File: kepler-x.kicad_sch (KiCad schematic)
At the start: 60 parts, among them IC1 SLG46826G, J1 HDMI_C_1.3, J2 HDMI_A, J3 Jack_3.5mm_3pin, J4 RasPI_IO_Header_B+, SW1 SWITCH_INV, SW2 SWITCH_INV, U1 Bus-X68000-ext, U10 74AHC16374, U11 74LVTH162245, U12 TC7MPB9307F, U13 TC7MPB9307F, U14 P0082(DE0-NANO), U15 PLR135-T10, U16 PCM5102, U17 LT1117-3.3, U2 LT1117-3.3, U3 INA3221, U4 74AHC16374, U5 74AHC16374, U6 WM8804GEDS{slash}RV, U7 74AHC16374, U8 74AHC16374, U9 74AHC16374, X1 SG-8002DC(24.576MHz), X2 ASV-xxxMHz, Y1 12MHz

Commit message: Today's version
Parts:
- removed J2: HDMI_A, Connector_HDMI:HDMI_A_Kycon_KDMIX-SL1-NS-WS-B15_VerticalRightAngle, symbol Connector:HDMI_A
- added H1, H2: MountingHole, MountingHole:MountingHole_3.7mm, symbol Mechanical:MountingHole
- added H3, H4: MountingHole, MountingHole:MountingHole_2.7mm_M2.5, symbol Mechanical:MountingHole
- added J2: USB_B_Micro, symbol Connector:USB_B_Micro
- added J5, J6: Jack_3.5mm_3pin, Connector_Audio:Jack_3.5mm_Switronic_ST-005-G_horizontal, symbol w_connectors:Jack_3.5mm_3pin
- C10, C6, C7, C8, C9: footprint Capacitor_SMD:C_0603_1608Metric -> Capacitor_SMD:C_0603_1608Metric_Pad1.08x0.95mm_HandSolder
- C3, C4: footprint Capacitor_THT:CP_Radial_D5.0mm_P2.50mm -> Capacitor_SMD:C_0603_1608Metric_Pad1.08x0.95mm_HandSolder
- J3: footprint Connector_Audio:Jack_3.5mm_CUI_SJ-3523-SMT_Horizontal -> Connector_Audio:Jack_3.5mm_Switronic_ST-005-G_horizontal
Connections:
- net ExAB1: now also U9.3 (1Q2); no longer U9.22 (2Q7)
- net ExAB10: now also U9.16 (2Q3); no longer U9.9 (1Q6)
- net ExAB11: now also U9.17 (2Q4); no longer U9.8 (1Q5)
- net ExAB12: now also U9.19 (2Q5); no longer U9.6 (1Q4)
- net ExAB13: now also U9.20 (2Q6); no longer U9.5 (1Q3)
- net ExAB14: now also U9.22 (2Q7); no longer U9.3 (1Q2)
- net ExAB15: now also U9.23 (2Q8); no longer U9.2 (1Q1)
- net ExAB16: now also U8.2 (1Q1); no longer U8.23 (2Q8)
- net ExAB17: now also U8.3 (1Q2); no longer U8.22 (2Q7)
- net ExAB18: now also U8.5 (1Q3); no longer U8.20 (2Q6)
- net ExAB19: now also U8.6 (1Q4); no longer U8.19 (2Q5)
- net ExAB2: now also U9.5 (1Q3); no longer U9.20 (2Q6)
- net ExAB20: now also U8.8 (1Q5); no longer U8.17 (2Q4)
- net ExAB21: now also U8.9 (1Q6); no longer U8.16 (2Q3)
- net ExAB22: now also U8.11 (1Q7); no longer U8.14 (2Q2)
- net ExAB23: now also U8.12 (1Q8); no longer U8.13 (2Q1)
- net ExAB3: now also U9.6 (1Q4); no longer U9.19 (2Q5)
- net ExAB4: now also U9.8 (1Q5); no longer U9.17 (2Q4)
- net ExAB5: now also U9.9 (1Q6); no longer U9.16 (2Q3)
- net ExAB6: now also U9.11 (1Q7); no longer U9.14 (2Q2)
- net ExAB7: now also U9.12 (1Q8); no longer U9.13 (2Q1)
- net ExAB8: now also U9.13 (2Q1); no longer U9.12 (1Q8)
- net ExAB9: now also U9.14 (2Q2); no longer U9.11 (1Q7)
- net ExDB0: now also U10.2 (1Q1); no longer U10.23 (2Q8)
- net ExDB1: now also U10.3 (1Q2); no longer U10.22 (2Q7)
- net ExDB10: now also U10.16 (2Q3); no longer U10.9 (1Q6)
- net ExDB11: now also U10.17 (2Q4); no longer U10.8 (1Q5)
- net ExDB12: now also U10.19 (2Q5); no longer U10.6 (1Q4)
- net ExDB13: now also U10.20 (2Q6); no longer U10.5 (1Q3)
- net ExDB14: now also U10.22 (2Q7); no longer U10.3 (1Q2)
- net ExDB15: now also U10.23 (2Q8); no longer U10.2 (1Q1)
- net ExDB2: now also U10.5 (1Q3); no longer U10.20 (2Q6)
- net ExDB3: now also U10.6 (1Q4); no longer U10.19 (2Q5)
- net ExDB4: now also U10.8 (1Q5); no longer U10.17 (2Q4)
- net ExDB5: now also U10.9 (1Q6); no longer U10.16 (2Q3)
- net ExDB6: now also U10.11 (1Q7); no longer U10.14 (2Q2)
- net ExDB7: now also U10.12 (1Q8); no longer U10.13 (2Q1)
- net ExDB8: now also U10.13 (2Q1); no longer U10.12 (1Q8)
- net ExDB9: now also U10.14 (2Q2); no longer U10.11 (1Q7)
- net ExFC0: now also U8.13 (2Q1); no longer U8.12 (1Q8)
- net ExFC1: now also U8.14 (2Q2); no longer U8.11 (1Q7)
- net ExFC2: now also U8.16 (2Q3); no longer U8.9 (1Q6)
- net GND: now also J2.5 (GND), J2.6 (Shield)
- net iB_AO_OE: no longer U9.1 (1~{OE})
- net iSB0: now also U10.47 (1D1), U8.47 (1D1), U9.47 (1D1); no longer U10.26 (2D8), U8.26 (2D8), U9.26 (2D8)
- net iSB1: now also U10.46 (1D2), U8.46 (1D2), U9.46 (1D2); no longer U10.27 (2D7), U8.27 (2D7), U9.27 (2D7)
- net iSB10: now also U10.33 (2D3), U8.33 (2D3), U9.33 (2D3); no longer U10.40 (1D6), U8.40 (1D6), U9.40 (1D6)
- net iSB11: now also U10.32 (2D4), U8.32 (2D4), U9.32 (2D4); no longer U10.41 (1D5), U8.41 (1D5), U9.41 (1D5)
- net iSB12: now also U10.30 (2D5), U8.30 (2D5), U9.30 (2D5); no longer U10.43 (1D4), U8.43 (1D4), U9.43 (1D4)
- net iSB13: now also U10.29 (2D6), U8.29 (2D6), U9.29 (2D6); no longer U10.44 (1D3), U8.44 (1D3), U9.44 (1D3)
- net iSB14: now also U10.27 (2D7), U8.27 (2D7), U9.27 (2D7); no longer U10.46 (1D2), U8.46 (1D2), U9.46 (1D2)
- net iSB15: now also U10.26 (2D8), U8.26 (2D8), U9.26 (2D8); no longer U10.47 (1D1), U8.47 (1D1), U9.47 (1D1)
- net iSB2: now also U10.44 (1D3), U8.44 (1D3), U9.44 (1D3); no longer U10.29 (2D6), U8.29 (2D6), U9.29 (2D6)
- net iSB3: now also U10.43 (1D4), U8.43 (1D4), U9.43 (1D4); no longer U10.30 (2D5), U8.30 (2D5), U9.30 (2D5)
- net iSB4: now also U10.41 (1D5), U8.41 (1D5), U9.41 (1D5); no longer U10.32 (2D4), U8.32 (2D4), U9.32 (2D4)
- net iSB5: now also U10.40 (1D6), U8.40 (1D6), U9.40 (1D6); no longer U10.33 (2D3), U8.33 (2D3), U9.33 (2D3)
- net iSB6: now also U10.38 (1D7), U8.38 (1D7), U9.38 (1D7); no longer U10.35 (2D2), U8.35 (2D2), U9.35 (2D2)
- net iSB7: now also U10.37 (1D8), U8.37 (1D8), U9.37 (1D8); no longer U10.36 (2D1), U8.36 (2D1), U9.36 (2D1)
- net iSB8: now also U10.36 (2D1), U8.36 (2D1), U9.36 (2D1); no longer U10.37 (1D8), U8.37 (1D8), U9.37 (1D8)
- net iSB9: now also U10.35 (2D2), U8.35 (2D2), U9.35 (2D2); no longer U10.38 (1D7), U8.38 (1D7), U9.38 (1D7)
- net at R1.1, U1.A49 (VCC1), U1.A50 (VCC1)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: now also J2.1 (VBUS)
- no-connect marks 57 -> 54
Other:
- moved on the sheet: D1, U10, U8, U9

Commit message: Today's version
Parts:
- removed J2: USB_B_Micro, symbol Connector:USB_B_Micro
- added D3, D4, D5: Led_Small, symbol device:Led_Small
- added J2, J7: Conn_01x02_Male, symbol Connector:Conn_01x02_Male
- added JP4, JP5: Jumper_NC_Small, symbol device:Jumper_NC_Small
- added R6, R7, R9: 1K, symbol Device:R_Small_US
- added R8: 10K, symbol Device:R_Small_US
- added RP7: R_PACK4, Resistor_SMD:R_Array_Convex_4x0603, symbol device:R_PACK4
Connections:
- net I2C_SCK is gone; now on net I2C_SCL: U14.JP1_7 (GPIO_04)
- net i2C_SCL is gone; now on net I2C_SCL: JP1.2, JP2.2
- net +3V3: now also U3.16 (VPU), U3.4 (VS), R8.1, RP7.5 (R4), RP7.6 (R3), RP7.7 (R2), RP7.8 (R1)
- net ExBGACK: now also U1.B48 (~{BGACK}); no longer U1.B47 (~{BG})
- net GND: now also U16.10 (DEMP), U16.11 (FLT), U16.16 (FMT), J2.2 (Pin_2), J7.2 (Pin_2), JP4.2, R6.2, R7.2, R9.2
- net I2C_SCL: now also U3.6 (SCL), U6.1 (SCLK)
- net I2C_SDA: now also U3.7 (SDA), U6.3 (SDIN/HWMODE), R8.2
- net VCC: no longer U3.4 (VS)
- net iB_AO_OE: now also U9.1 (1~{OE})
- net iCLK24M576: now also JP5.1; no longer X2.3 (OUT)
- net iEXRESET: now also U6.6 (RESETB)
- net at R1.1, U1.A49 (VCC1), U1.A50 (VCC1)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: now also J2.1 (Pin_1), J7.1 (Pin_1)
- net at U6.2 (GPO0/SWIFMODE): now also D3.2 (A)
- net at U6.4 (SDOUT/GPO2): now also D5.2 (A)
- net at U6.5 (CSB/GPO1): now also D4.2 (A)
- net at U3.10 (PV): now also RP7.4 (P4)
- net at U3.13 (TC): now also RP7.1 (P1)
- net at U3.5 (A0): now also JP4.1
- net at U3.8 (WARN): now also RP7.2 (P2)
- net at U3.9 (CRIT): now also RP7.3 (P3)
- net at TR1.4 (NC): no longer TR1.5 (NC)
- new net: JP5.2, X2.3 (OUT)
- new net: D4.1 (K), R7.1
- new net: D5.1 (K), R9.1
- new net: D3.1 (K), R6.1
- no-connect marks 54 -> 75
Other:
- moved on the sheet: C1, C10, C2, C3, C4, C5, C6, J4, J5, J6, R1, R2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

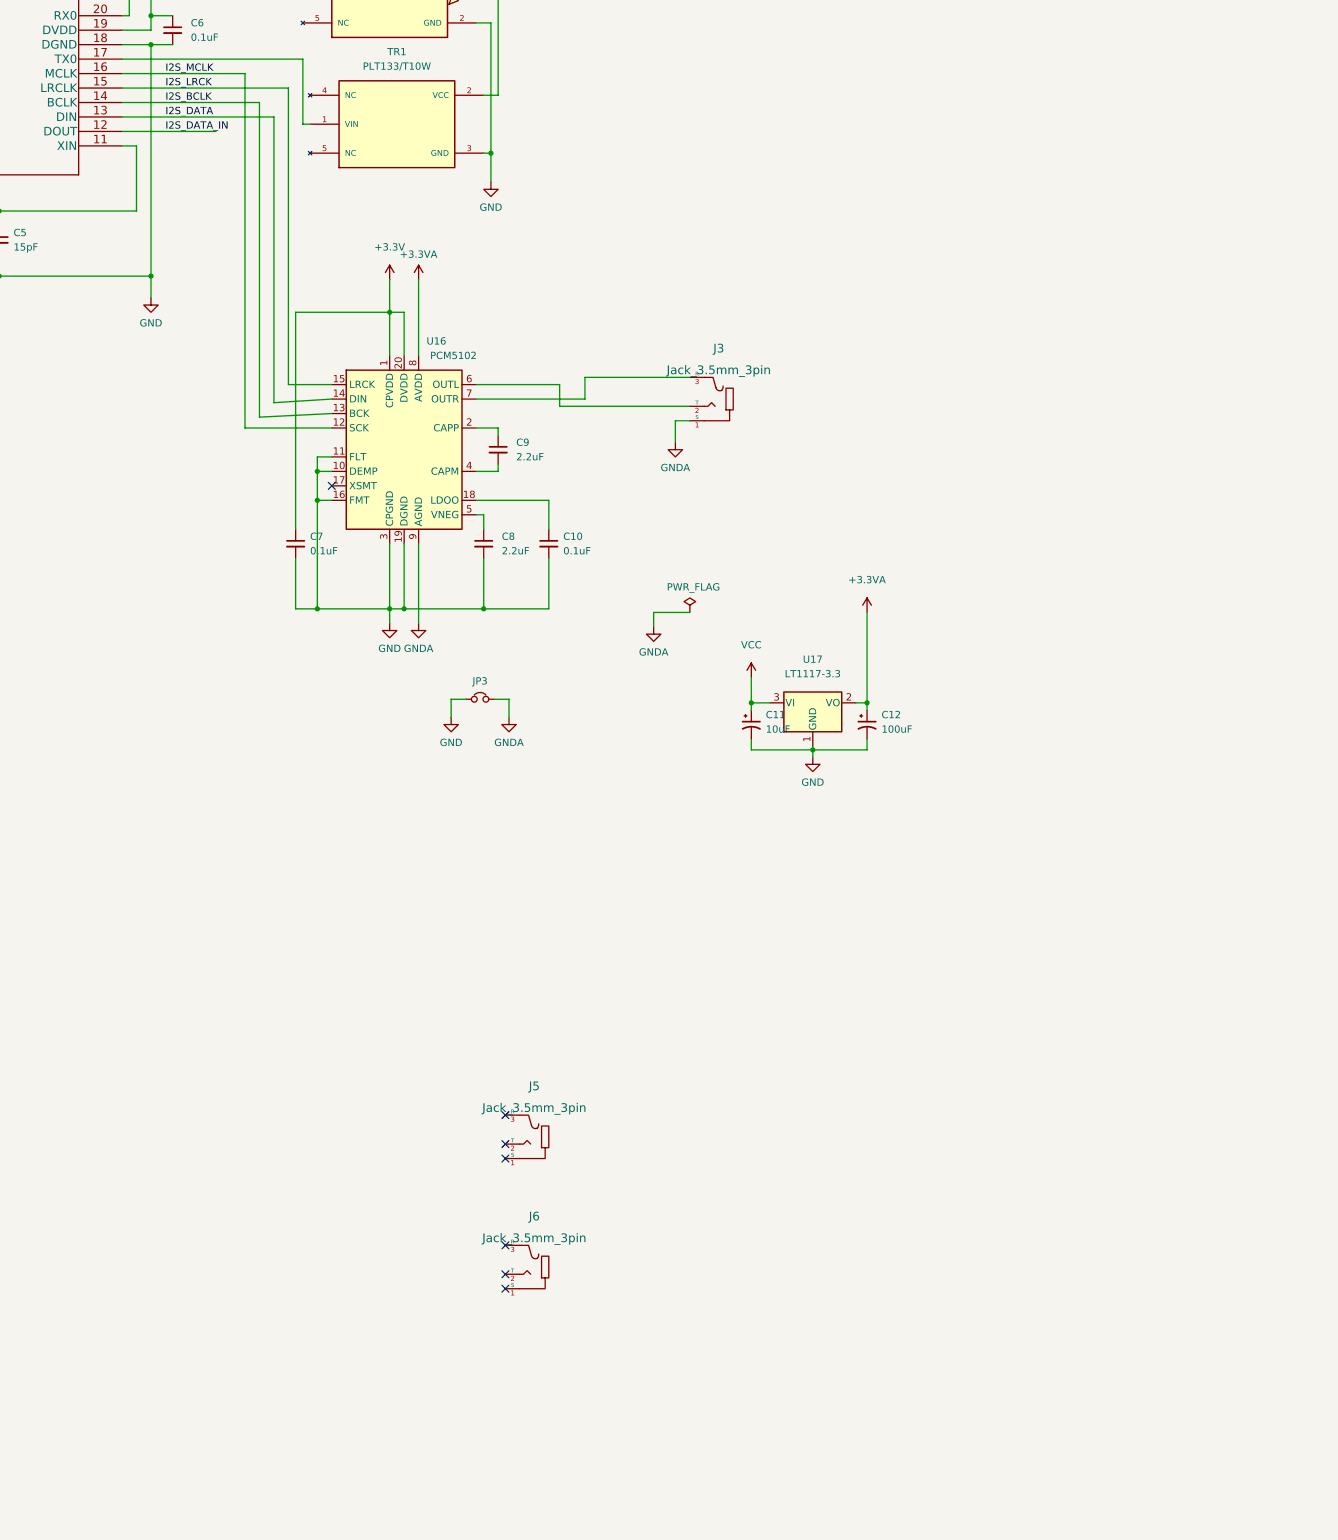
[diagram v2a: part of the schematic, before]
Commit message: Today's version
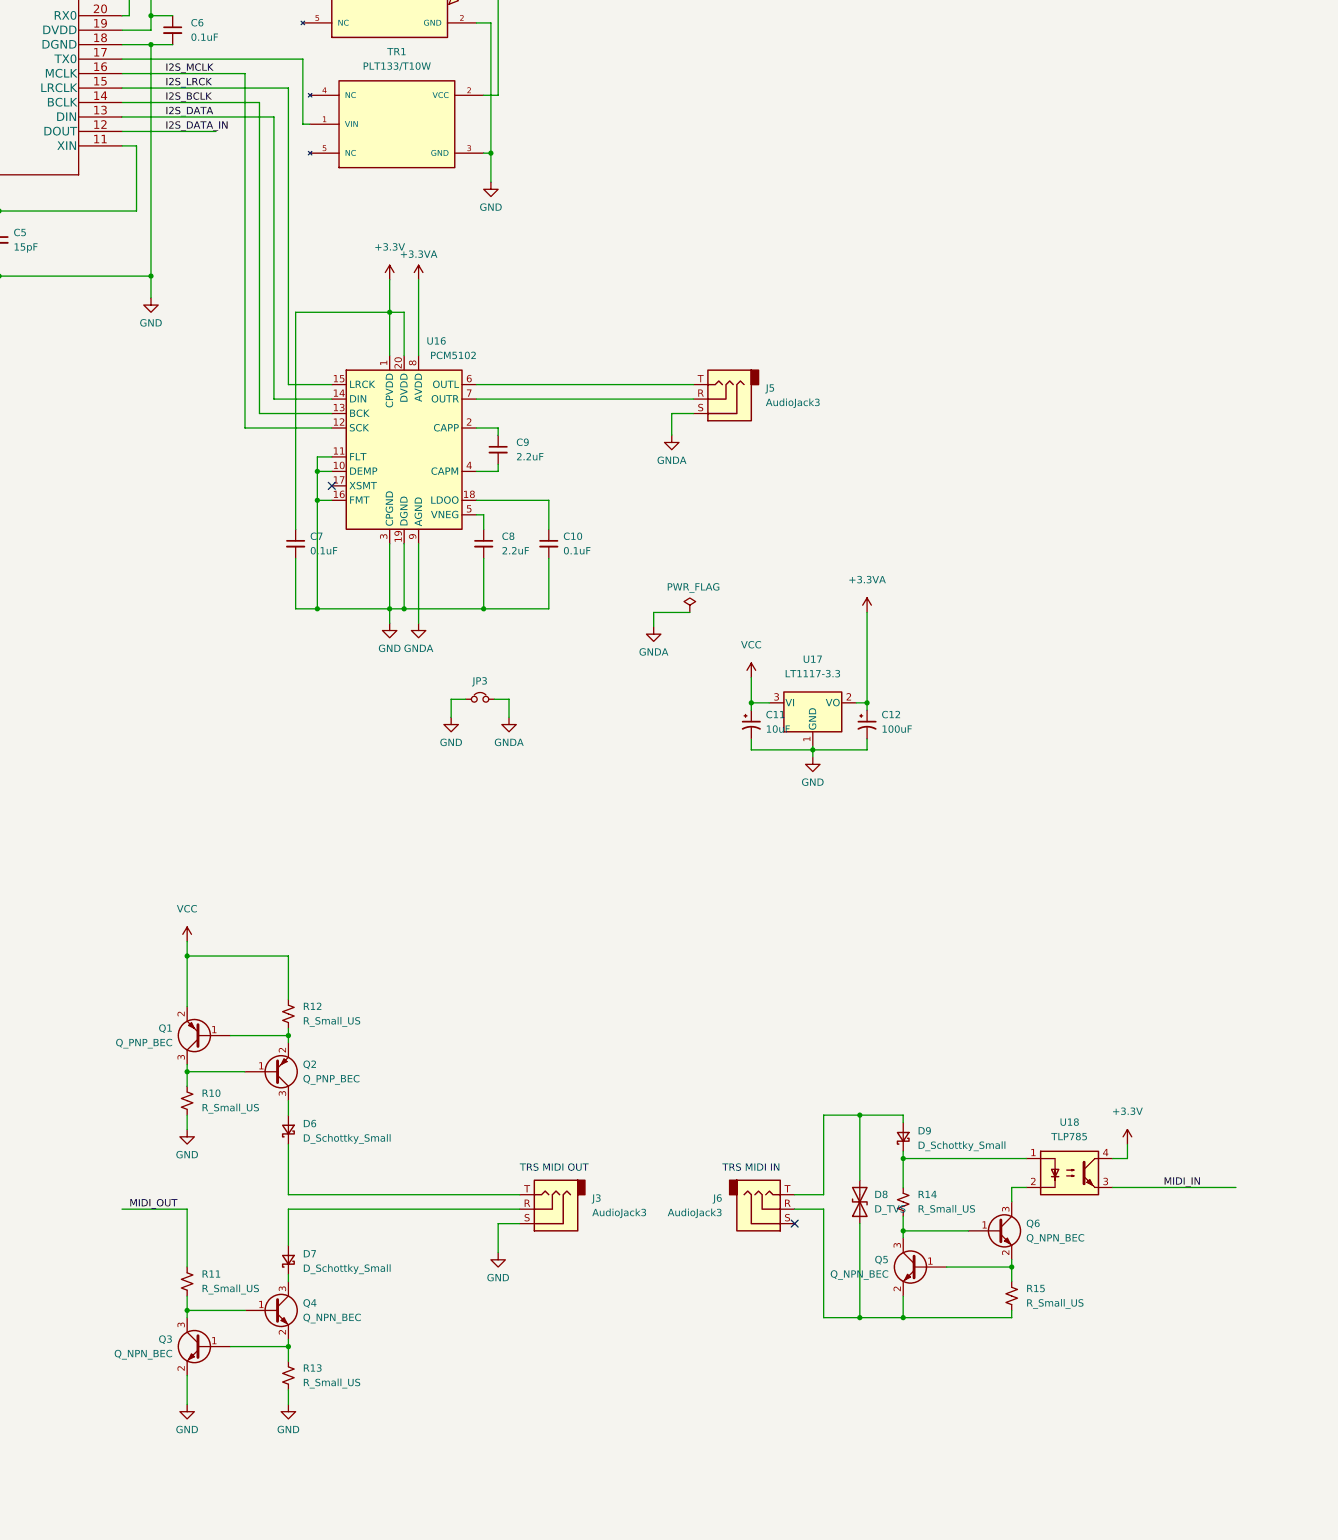
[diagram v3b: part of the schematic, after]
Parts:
- removed J3, J5, J6: Jack_3.5mm_3pin, Connector_Audio:Jack_3.5mm_Switronic_ST-005-G_horizontal, symbol w_connectors:Jack_3.5mm_3pin
- added D6, D7, D9: D_Schottky_Small, Diode_SMD:D_1206_3216Metric_Pad1.42x1.75mm_HandSolder, symbol Device:D_Schottky_Small
- added D8: D_TVS, Diode_SMD:D_1206_3216Metric_Pad1.42x1.75mm_HandSolder, symbol Device:D_TVS
- added J3, J5, J6: AudioJack3, Connector_Audio:Jack_3.5mm_Switronic_ST-005-G_horizontal, symbol Connector:AudioJack3
- added Q1, Q2: Q_PNP_BEC, Package_TO_SOT_SMD:SC-59_Handsoldering, symbol Device:Q_PNP_BEC
- added Q3, Q4, Q5, Q6: Q_NPN_BEC, Package_TO_SOT_SMD:SC-59_Handsoldering, symbol Device:Q_NPN_BEC
- added R10, R11, R12, R13, R14, R15: R_Small_US, Resistor_SMD:R_0603_1608Metric_Pad0.98x0.95mm_HandSolder, symbol Device:R_Small_US
- added U18: TLP785, Package_DIP:DIP-4_W7.62mm, symbol Isolator:TLP785
- D1, D2: footprint Diode_SMD:D_MELF_Handsoldering -> Diode_SMD:D_1206_3216Metric_Pad1.42x1.75mm_HandSolder
- D3, D4, D5: footprint (none) -> LED_SMD:LED_0603_1608Metric_Pad1.05x0.95mm_HandSolder
- J2, J7: footprint (none) -> Connector_PinHeader_2.54mm:PinHeader_1x02_P2.54mm_Vertical
- JP4: footprint (none) -> digikey-footprints:PinHeader_1x2_P2.54mm
- JP5: footprint (none) -> Jumper:SolderJumper-2_P1.3mm_Bridged_RoundedPad1.0x1.5mm
- R6, R7, R8, R9: footprint (none) -> Resistor_SMD:R_0603_1608Metric_Pad0.98x0.95mm_HandSolder
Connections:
- net +3V3: now also U18.4
- net GND: now also J3.S, Q3.2 (E), R10.2, R13.2
- net GNDA: now also J5.S
- net MIDI_IN: now also U18.3
- net MIDI_OUT: now also R11.1
- net VCC: now also Q1.2 (E), R12.1
- net at U16.6 (OUTL): now also J5.T
- net at U16.7 (OUTR): now also J5.R
- new net: D7.2 (A), J3.R
- new net: D6.1 (K), J3.T
- new net: Q3.3 (C), Q4.1 (B), R11.2
- new net: Q1.1 (B), Q2.2 (E), R12.2
- new net: Q1.3 (C), Q2.1 (B), R10.1
- new net: Q5.1 (B), Q6.2 (E), R15.1
- new net: D8.1 (A1), J6.R, Q5.2 (E), R15.2
- new net: Q3.1 (B), Q4.2 (E), R13.1
- new net: D9.1 (K), R14.1, U18.1
- new net: Q5.3 (C), Q6.1 (B), R14.2
- new net: Q6.3 (C), U18.2
- new net: D7.1 (K), Q4.3 (C)
- new net: D6.2 (A), Q2.3 (C)
- new net: D8.2 (A2), D9.2 (A), J6.T
- no-connect marks 75 -> 70
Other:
- note added: "TRS MIDI IN"
- note added: "TRS MIDI OUT"
